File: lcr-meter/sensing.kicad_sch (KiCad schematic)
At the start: 6 parts, among them J4 Conn_01x04, U10 AMP03GPZ, U2 AMP03GPZ, U21 AMP03GPZ, U3 AMP03GPZ

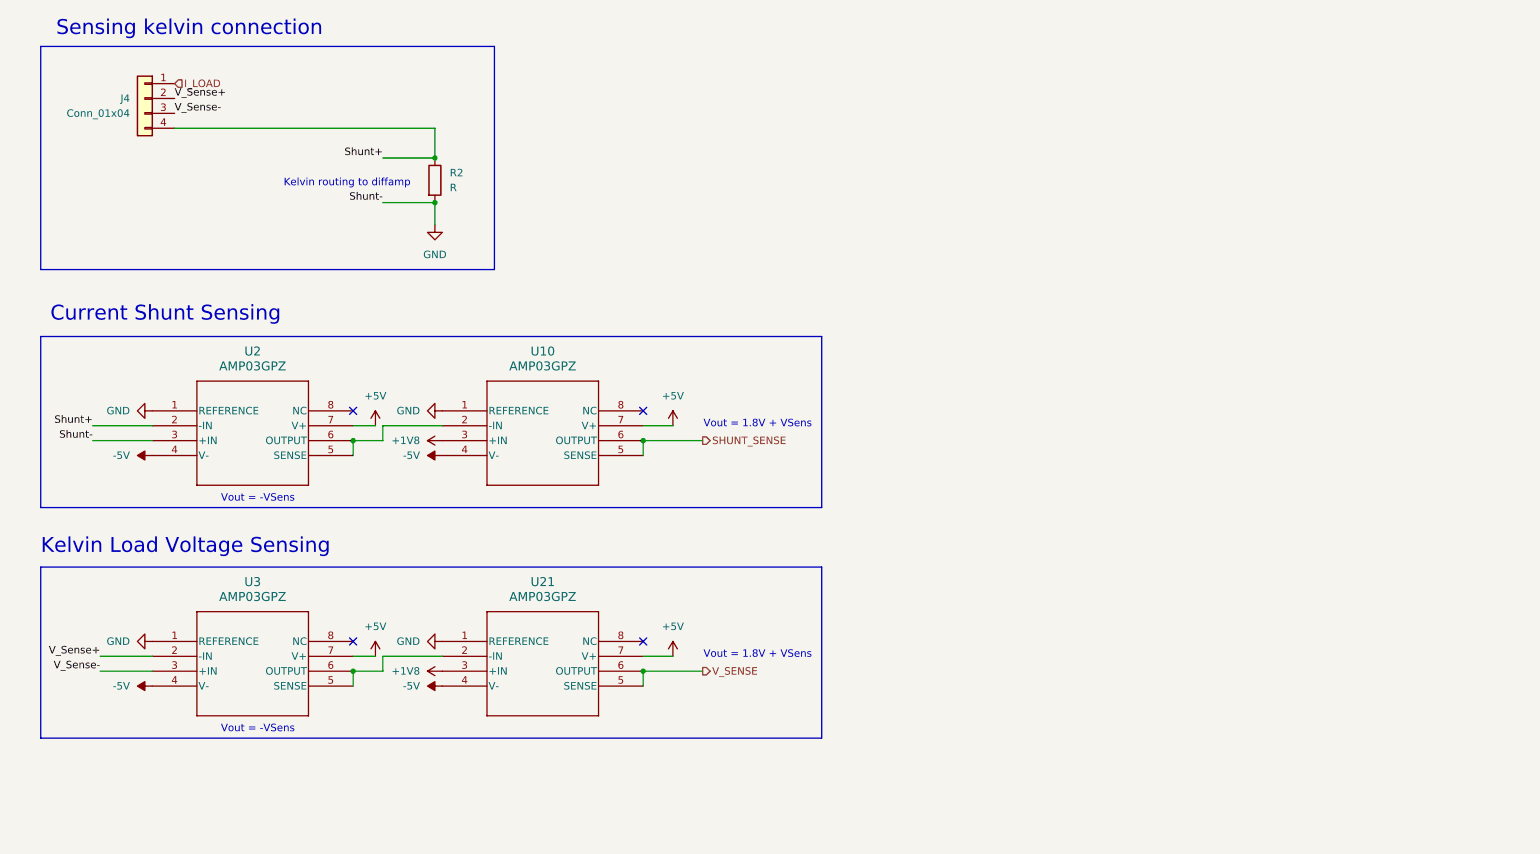
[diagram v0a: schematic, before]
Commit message: Schematic polishing
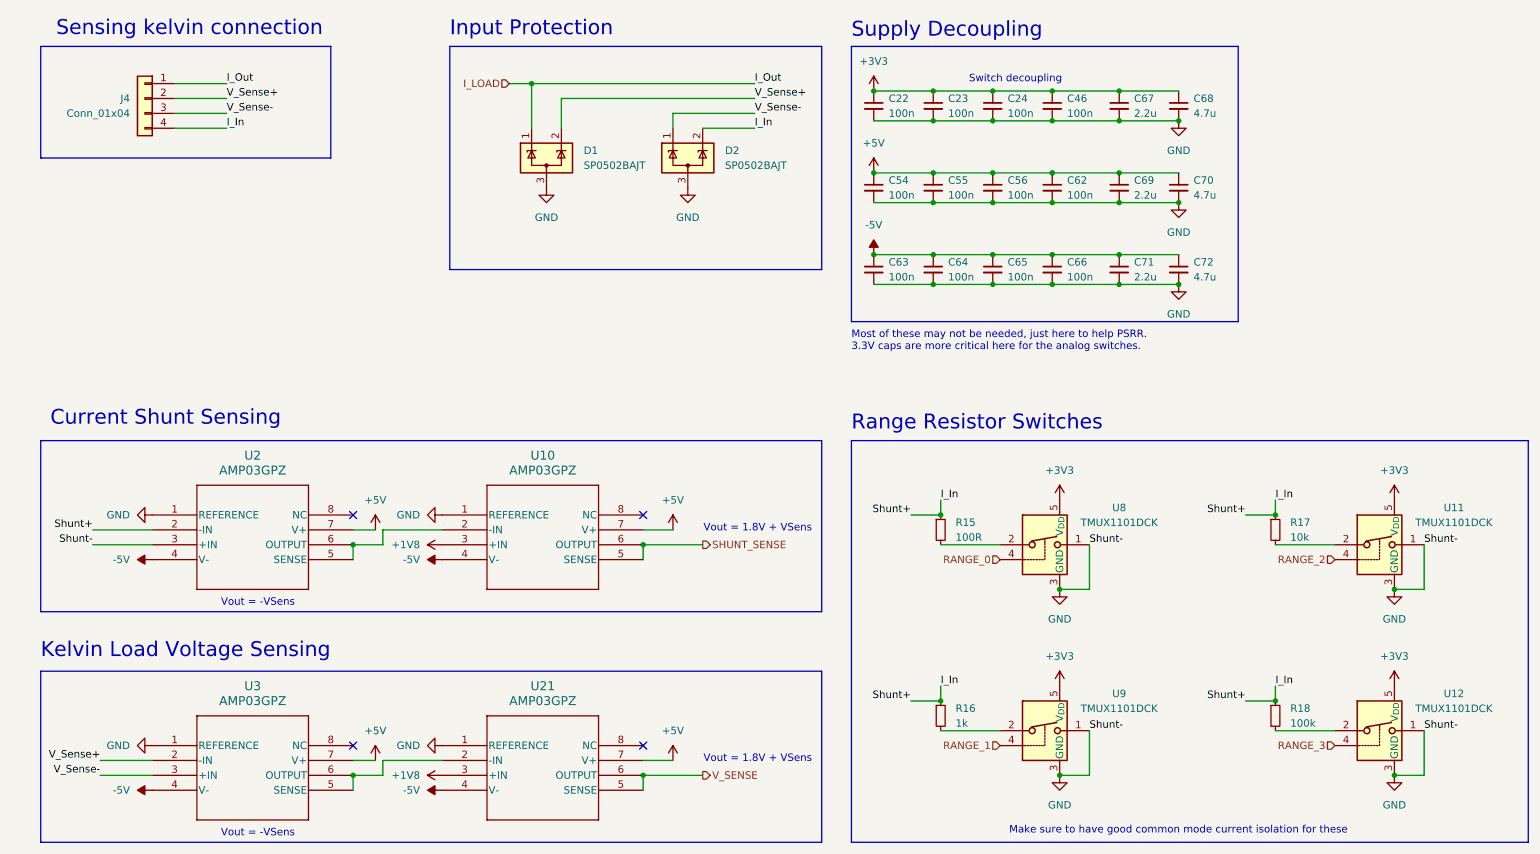
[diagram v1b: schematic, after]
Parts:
- removed R2: R, symbol Device:R
- added C22, C23, C24, C46, C54, C55, C56, C62, C63, C64, C65, C66: 100n, Capacitor_SMD:C_0402_1005Metric, symbol Device:C_Small
- added C67, C69, C71: 2.2u, Capacitor_SMD:C_0402_1005Metric, symbol Device:C_Small
- added C68, C70, C72: 4.7u, Capacitor_SMD:C_0402_1005Metric, symbol Device:C_Small
- added D1, D2: SP0502BAJT, Package_TO_SOT_SMD:SOT-323_SC-70, symbol Power_Protection:SP0502BAJT
- added R15: 100R, Resistor_SMD:R_0402_1005Metric, symbol Device:R_Small
- added R16: 1k, Resistor_SMD:R_0402_1005Metric, symbol Device:R_Small
- added R17: 10k, Resistor_SMD:R_0402_1005Metric, symbol Device:R_Small
- added R18: 100k, Resistor_SMD:R_0402_1005Metric, symbol Device:R_Small
- added U11, U12, U8, U9: TMUX1101DCK, Package_TO_SOT_SMD:SOT-23-5, symbol Analog_Switch:TMUX1101DCK
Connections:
- net +5V: now also C54.1, C55.1, C56.1, C62.1, C69.1, C70.1
- net -5V: now also C63.1, C64.1, C65.1, C66.1, C71.1, C72.1
- net GND: now also C22.2, C23.2, C24.2, C46.2, C54.2, C55.2, C56.2, C62.2, C63.2, C64.2, C65.2, C66.2, C67.2, C68.2, C69.2, C70.2, C71.2, C72.2, D1.3 (A), D2.3 (A), U11.1, U11.3 (GND), U12.1, U12.3 (GND), U8.1, U8.3 (GND), U9.1, U9.3 (GND)
- net I_LOAD: now also D1.1 (K)
- net V_Sense+: now also D1.2 (K)
- net V_Sense-: now also D2.1 (K)
- net Shunt+ renamed I_In
- net I_In: now also D2.2 (K), R15.1, R16.1, R17.1, R18.1
- new net: R15.2, U8.2
- new net: R18.2, U12.2
- new net: R16.2, U9.2
- new net: R17.2, U11.2
- new net +3V3: C22.1, C23.1, C24.1, C46.1, C67.1, C68.1, U11.5 (V_{DD}), U12.5 (V_{DD}), U8.5 (V_{DD}), U9.5 (V_{DD})
- new net RANGE_0: U8.4
- new net RANGE_1: U9.4
- new net RANGE_2: U11.4
- new net RANGE_3: U12.4
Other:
- note added: "Input Protection"
- note added: "Make sure to have good common mode current isolation for these"
- note added: "Most of these may not be needed, just here to help PSRR. 3.3V caps are more critical here for the analog switches."
- note added: "Range Resistor Switches"
- note added: "Supply Decoupling"
- note added: "Switch decoupling"
- note removed: "Kelvin routing to diffamp"
- moved on the sheet: U10, U2, U21, U3

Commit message: Schematic polishing
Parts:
- C68, C70, C72: footprint Capacitor_SMD:C_0402_1005Metric -> Capacitor_SMD:C_0805_2012Metric
- J4: footprint (none) -> Connector_PinHeader_2.54mm:PinHeader_1x04_P2.54mm_Vertical
- U10, U2, U21, U3: footprint N_8_ADI -> footprints:N_8_ADI
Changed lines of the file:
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@@
 			)
 		)
-		(property "Footprint" "N_8_ADI"
+		(property "Footprint" "footprints:N_8_ADI"
 			(at 41.91 144.78 0)
 			(effects
@@
 			)
 		)
-		(property "Footprint" "Capacitor_SMD:C_0402_1005Metric"
+		(property "Footprint" "Capacitor_SMD:C_0805_2012Metric"
 			(at 217.17 63.5 0)
 			(effects
@@
 			)
 		)
-		(property "Footprint" "N_8_ADI"
+		(property "Footprint" "footprints:N_8_ADI"
 			(at 91.44 105.41 0)
 			(effects
@@
 			)
 		)
-		(property "Footprint" ""
+		(property "Footprint" "Connector_PinHeader_2.54mm:PinHeader_1x04_P2.54mm_Vertical"
 			(at 40.64 34.29 0)
 			(effects
@@
 			)
 		)
-		(property "Footprint" "N_8_ADI"
+		(property "Footprint" "footprints:N_8_ADI"
 			(at 41.91 105.41 0)
 			(effects
@@
 			)
 		)
-		(property "Footprint" "Capacitor_SMD:C_0402_1005Metric"
+		(property "Footprint" "Capacitor_SMD:C_0805_2012Metric"
 			(at 217.17 49.53 0)
 			(effects
@@
 			)
 		)
-		(property "Footprint" "Capacitor_SMD:C_0402_1005Metric"
+		(property "Footprint" "Capacitor_SMD:C_0805_2012Metric"
 			(at 217.17 35.56 0)
 			(effects
@@
 			)
 		)
-		(property "Footprint" "N_8_ADI"
+		(property "Footprint" "footprints:N_8_ADI"
 			(at 91.44 144.78 0)
 			(effects
